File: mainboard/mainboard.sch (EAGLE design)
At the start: 27 parts, among them J1 BATTERY_CONNDEANS, P1 IMU, P2 analogin, P3 analogin, P4 I2C, U1 DWM1000, U2 ESP8266, X1 04-JST-B4B-XH-A, X2 04-JST-B4B-XH-A

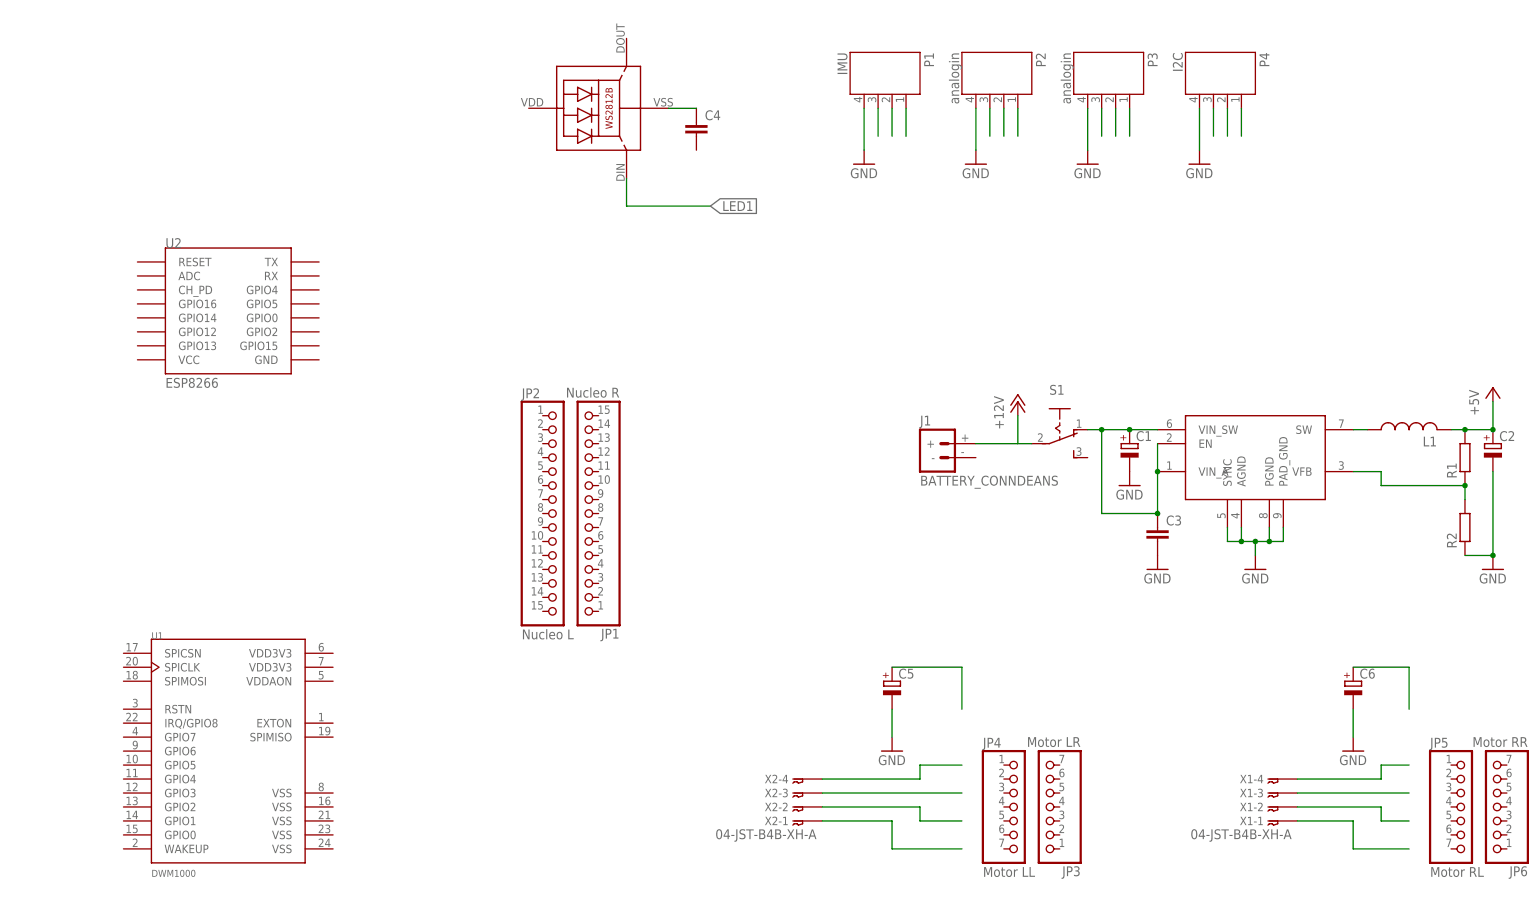
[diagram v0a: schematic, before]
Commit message: fit
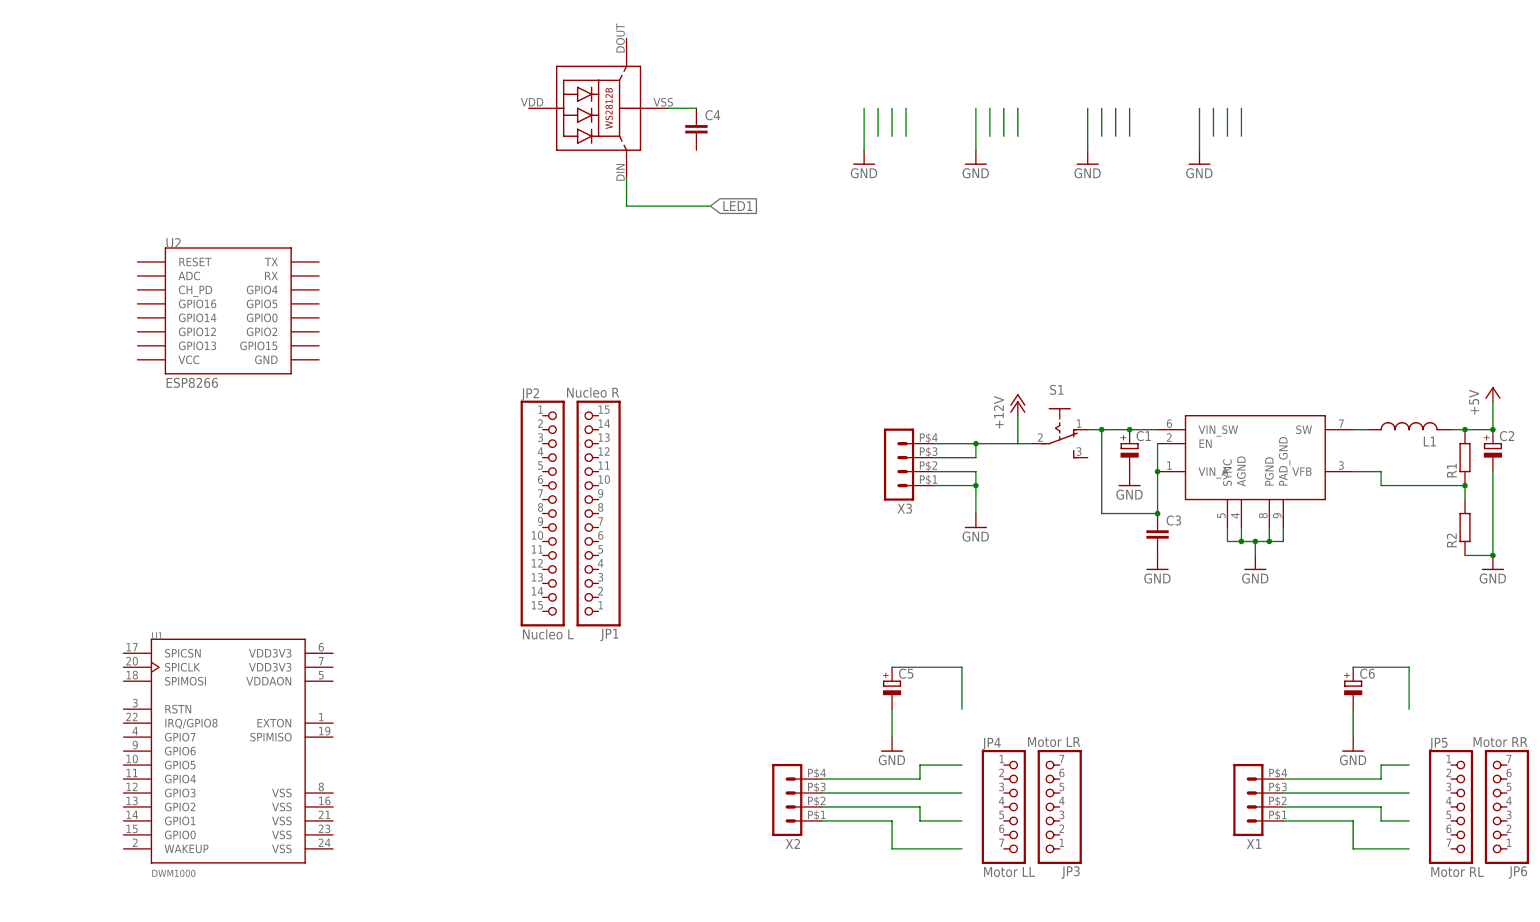
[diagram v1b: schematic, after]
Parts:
- removed J1: BATTERY_CONNDEANS, SparkFun-Connectors:BATTERY_CONNDEANS
- removed P1: IMU, jst-ph:JST-PH4
- removed P2, P3: analogin, jst-ph:JST-PH4
- removed P4: I2C, jst-ph:JST-PH4
- added X3: (no value), con-molex-micro-fit-3_0:HEADER_POS4_43045-0415
- X1, X2: value 04-JST-B4B-XH-A -> (none); device bt_con-jst-xh:04-JST-B4B-XH-A -> con-molex-micro-fit-3_0:HEADER_POS4_43045-0412
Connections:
- removed net N$1: P1.3
- removed net N$10: P3.3
- removed net N$11: P3.2
- removed net N$12: P3.1
- removed net N$13: P4.3
- removed net N$14: P4.2
- removed net N$15: P4.1
- removed net N$3: P1.2
- removed net N$6: P1.1
- removed net N$7: P2.3
- removed net N$8: P2.2
- removed net N$9: P2.1
- net +12V: now also X3.3, X3.4; no longer J1.+
- net GND: now also X3.1, X3.2; no longer P1.4, P2.4, P3.4, P4.4
- net N$19: now also X2.4; no longer X2-4.1
- net N$20: now also X2.3; no longer X2-3.1
- net N$21: now also X2.2; no longer X2-2.1
- net N$22: now also X2.1; no longer X2-1.1
- net N$23: now also X1.4; no longer X1-4.1
- net N$24: now also X1.3; no longer X1-3.1
- net N$25: now also X1.2; no longer X1-2.1
- net N$26: now also X1.1; no longer X1-1.1

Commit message: allparts
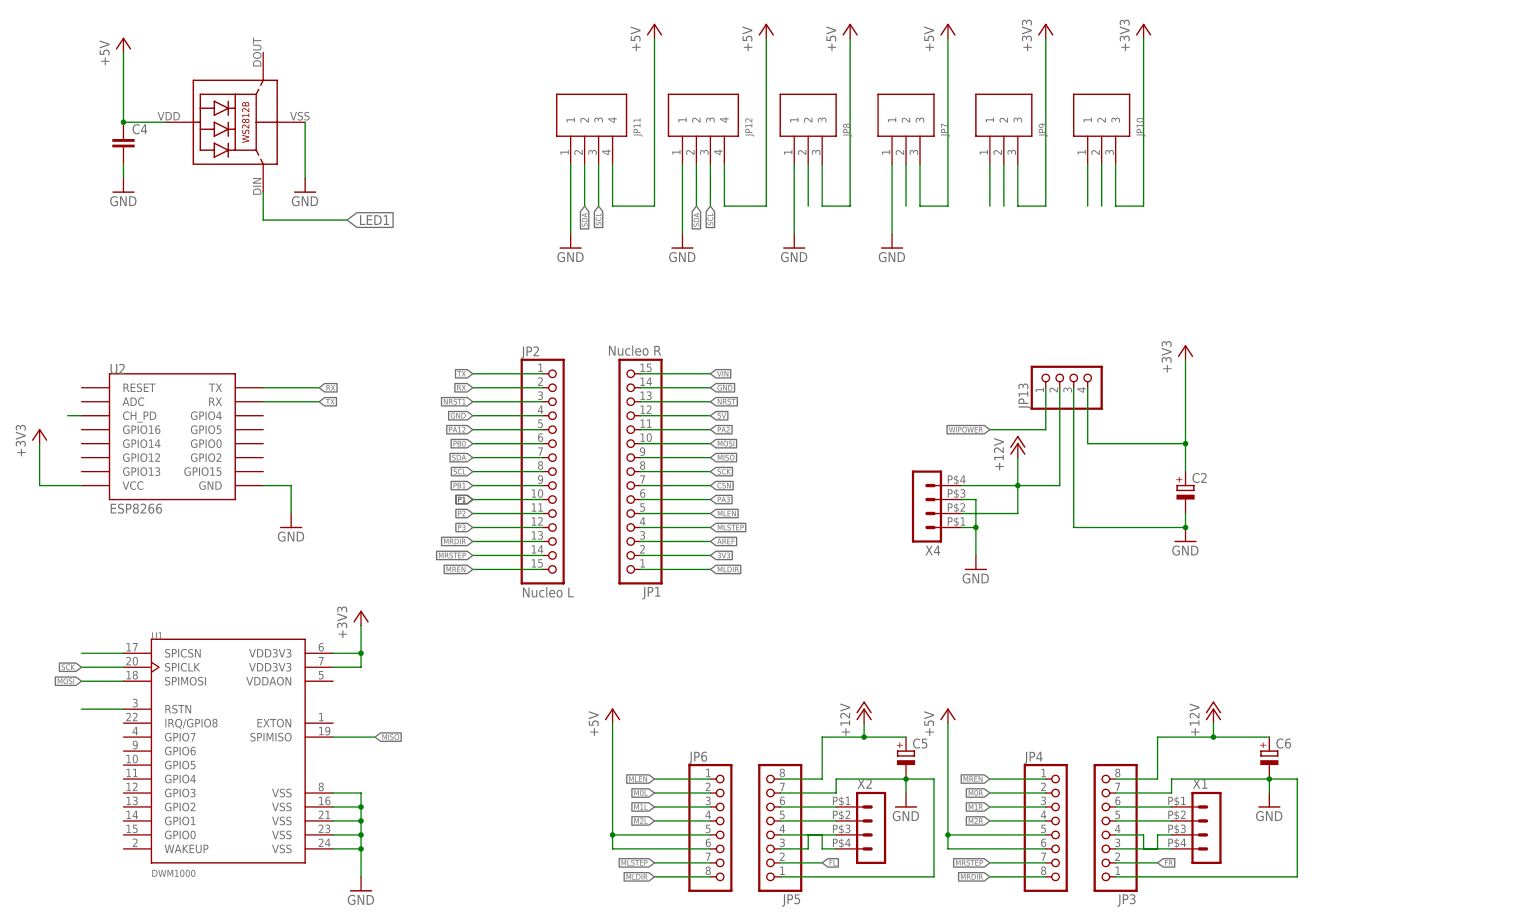
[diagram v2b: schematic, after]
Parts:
- removed C1: (no value), rcl:CPOL-EU153CLV-0405
- removed C3: (no value), rcl:C-EUC0603K
- removed L1: (no value), rcl:L-USL4035M
- removed R1, R2: (no value), rcl:R-EU_R0603
- removed S1: (no value), switch:255SB
- removed U$1: ST1S10PHR, ST1S10PHR:ST1S10PHR
- removed X3: (no value), con-molex-micro-fit-3_0:HEADER_POS4_43045-0415
- added JP10, JP7, JP8, JP9: 3PIN, jst_eph:3PIN
- added JP11, JP12: 4PIN, jst_eph:4PIN
- added JP13: (no value), pinhead-2:PINHD-1X04_2.54-SMD
- added X4: (no value), con-molex-micro-fit-3_0:HEADER_POS4_43045-0412
- JP3: value Motor LR -> (none); device pinhead-2:PINHD-1X07_2.54-SMD -> pinhead-2:PINHD-1X08_2.54-SMD
- JP4: value Motor LL -> (none); device pinhead-2:PINHD-1X07_2.54-SMD -> pinhead-2:PINHD-1X08_2.54-SMD
- JP5: value Motor RL -> (none); device pinhead-2:PINHD-1X07_2.54-SMD -> pinhead-2:PINHD-1X08_2.54-SMD
- JP6: value Motor RR -> (none); device pinhead-2:PINHD-1X07_2.54-SMD -> pinhead-2:PINHD-1X08_2.54-SMD
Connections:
- removed net N$16: C4.1, LED1.GND
- removed net N$17: C5.+
- removed net N$18: C6.+
- removed net N$4: R1.1, R2.2, U$1.VFB
- removed net N$5: C1.+, C3.1, S1.O, U$1.EN, U$1.VIN_A, U$1.VIN_SW
- new net +3V3: C2.+, JP10.3, JP13.4, JP9.3, U1.VDD3V3@1, U1.VDD3V3@2, U2.VCC
- new net 3V3: JP1.2
- new net 5V: JP1.12
- new net AREF: JP1.3
- new net CSN: JP1.7
- new net FL: JP5.2
- new net FR: JP3.2
- new net M0L: JP6.2
- new net M0R: JP4.2
- new net M1L: JP6.3
- new net M1R: JP4.3
- new net M2L: JP6.4
- new net M2R: JP4.4
- new net MISO: JP1.9, U1.SPIMISO
- new net MLDIR: JP1.1, JP6.8
- new net MLEN: JP1.5, JP6.1
- new net MLSTEP: JP1.4, JP6.7
- new net MOSI: JP1.10, U1.SPIMOSI
- new net MRDIR: JP2.13, JP4.8
- new net MREN: JP2.15, JP4.1
- new net MRSTEP: JP2.14, JP4.7
- new net N$1: JP9.1
- new net N$10: JP8.2
- new net N$12: JP3.6, X1.1
- new net N$13: JP7.2
- new net N$15: JP3.5, X1.2
- new net N$27: JP10.2
- new net N$3: JP9.2
- new net N$7: U1.SPICSN
- new net NRST: JP1.13
- new net NRST1: JP2.3
- new net P1: JP2.10
- new net P2: JP2.11
- new net P3: JP2.12
- new net PA12: JP2.5
- new net PA2: JP1.11
- new net PA3: JP1.6
- new net PB0: JP2.6
- new net PB1: JP2.9
- new net RX: JP2.2, U2.TX
- new net SCK: JP1.8, U1.SPICLK
- new net SCL: JP11.3, JP12.3, JP2.8
- new net SDA: JP11.2, JP12.2, JP2.7
- new net TX: JP2.1, U2.RX
- new net VIN: JP1.15
- new net WIPOWER: JP13.1
- net +12V: now also C5.+, C6.+, JP13.2, JP3.8, JP5.8, X4.2, X4.4; no longer S1.P, X3.3, X3.4
- net +5V: now also C4.1, JP11.4, JP12.4, JP4.5, JP4.6, JP6.5, JP6.6, JP7.3, JP8.3, LED1.VDD; no longer C2.+, L1.2, R1.2
- net GND: now also C4.2, JP1.14, JP11.1, JP12.1, JP13.3, JP2.4, JP3.1, JP3.7, JP5.1, JP5.7, JP7.1, JP8.1, LED1.GND, U1.VSS@1, U1.VSS@2, U1.VSS@3, U1.VSS@4, U1.VSS@5, U2.GND, X4.1, X4.3; no longer C1.-, C3.2, R2.1, U$1.AGND, U$1.PAD_GND, U$1.PGND, U$1.SYNC, X3.1, X3.2
- net N$19: now also JP3.4, X1.4; no longer X2.4
- net N$2: now also U2.CH_PD; no longer L1.1, U$1.SW
- net N$20: now also JP3.3, X1.3; no longer X2.3
- net N$21: now also JP5.6, X2.1; no longer X2.2
- net N$22: now also JP5.5, X2.2; no longer X2.1
- net N$23: now also JP5.4, X2.4; no longer X1.4
- net N$24: now also JP5.3, X2.3; no longer X1.3
- net N$25: now also U1.RSTN; no longer X1.2
- net N$26: now also JP10.1; no longer X1.1
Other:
- moved on the sheet: C2, C4, C5, C6, JP1, JP2, U2, X1, X2
